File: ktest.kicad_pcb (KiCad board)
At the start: 4 copper layers, 23.9 x 21.1 mm, 7 parts, among them J1 Conn_01x03_Pin

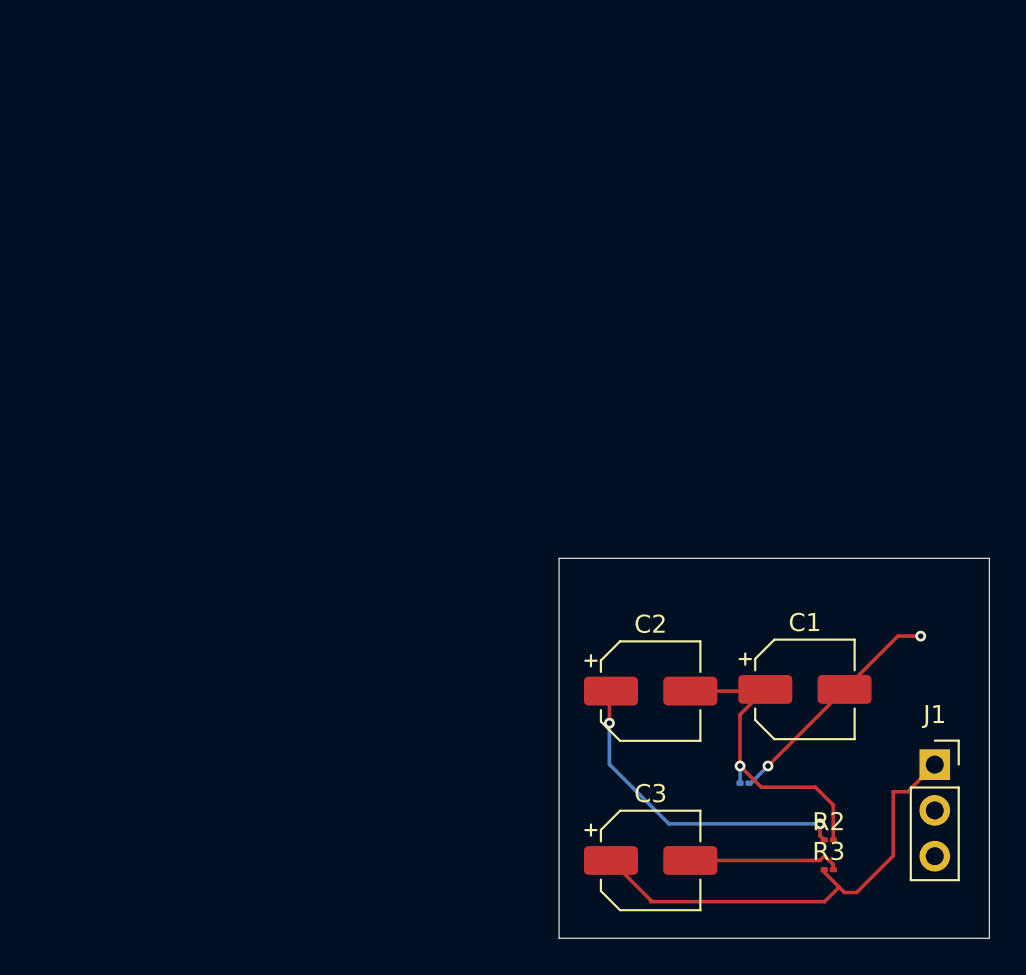
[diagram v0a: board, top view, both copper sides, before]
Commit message: Keep local changes
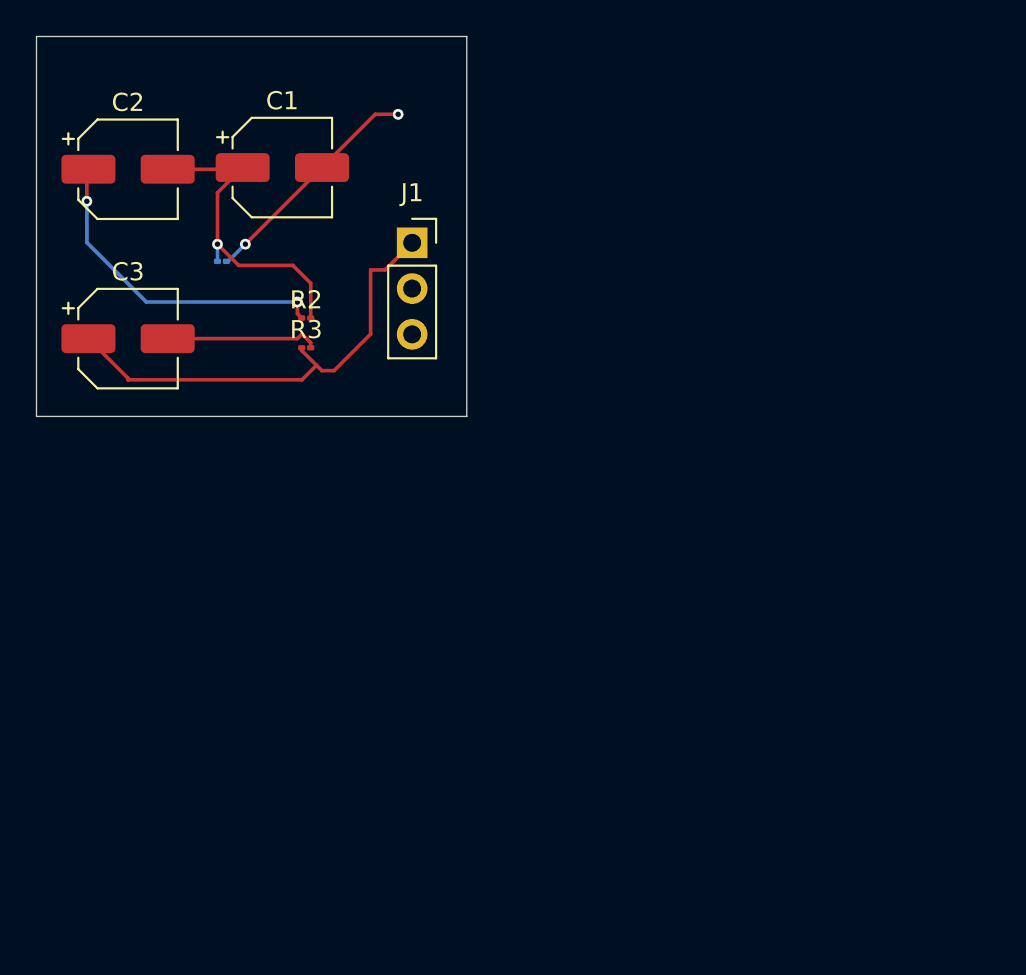
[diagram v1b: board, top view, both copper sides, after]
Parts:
- moved C2 41.0 mm to (97.5, 50.8)
- moved J1 41.0 mm to (113.3, 54.9)
- moved R1 41.0 mm to (102.7, 55.9)
- moved R2 41.0 mm to (107.4, 59.1)
- moved R3 41.0 mm to (107.4, 60.7)
- moved C3 41.0 mm to (97.5, 60.2)
- moved C1 41.0 mm to (106.1, 50.7)

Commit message: pdf assy image
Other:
- board text added: "angled bottom render"
- board text added: "angled top render"
- board text added: "bottom render"
- board text added: "top render"
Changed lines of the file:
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@@
 		(43 "User.3" user)
 		(45 "User.4" user)
+		(47 "User.5" user "AssemblyOverview")
+		(49 "User.6" user "AssemblyTop")
+		(51 "User.7" user "AssemblyBottom")
+		(53 "User.8" user)
 	)
 	(setup
@@
 		(capping no)
 		(filling no)
+		(zone_defaults)
 		(pcbplotparams
 			(layerselection 0x00000000_00000000_55555555_5755f5ff)
@@
 		(layer "Edge.Cuts")
 	)
+	(gr_rect
+		(start 40.132 39.624)
+		(end 77.724 75.946)
+		(stroke
+			(width 0.1)
+			(type default)
+		)
+		(fill no)
+		(layer "User.5")
+	)
+	(gr_rect
+		(start 126.746 40.005)
+		(end 164.338 76.327)
+		(stroke
+			(width 0.1)
+			(type default)
+		)
+		(fill no)
+		(layer "User.5")
+	)
+	(gr_rect
+		(start 139.954 51.054)
+		(end 174.752 85.598)
+		(stroke
+			(width 0.1)
+			(type default)
+		)
+		(fill no)
+		(layer "User.6")
+	)
+	(gr_rect
+		(start 133.096 36.322)
+		(end 161.29 68.072)
+		(stroke
+			(width 0.1)
+			(type default)
+		)
+		(fill no)
+		(layer "User.7")
+	)
+	(gr_text "angled top render"
+		(at 58.674 42.926 0)
+		(layer "User.5")
+		(effects
+			(font
+				(size 1 1)
+				(thickness 0.15)
+			)
+			(justify bottom)
+		)
+	)
+	(gr_text "angled bottom render"
+		(at 145.288 43.307 0)
+		(layer "User.5")
+		(effects
+			(font
+				(size 1 1)
+				(thickness 0.15)
+			)
+			(justify bottom)
+		)
+	)
+	(gr_text "top render"
+		(at 153.924 53.594 0)
+		(layer "User.6")
+		(effects
+			(font
+				(size 1 1)
+				(thickness 0.15)
+			)
+			(justify left bottom)
+		)
+	)
+	(gr_text "bottom render"
+		(at 141.986 38.862 0)
+		(layer "User.7")
+		(effects
+			(font
+				(size 1 1)
+				(thickness 0.15)
+			)
+			(justify left bottom)
+		)
+	)
 	(segment
 		(start 106.892 58.819)
@@
 		)
 	)
+	(group "kibot_image_blender_angled_bottom"
+		(members "47a33e86-0a7b-4fb2-9f1a-8c1f9bbd8aef" "e0f4d6b7-6642-4f52-86d4-2c7661283d27")
+	)
+	(group "kibot_image_blender_angled_top"
+		(members "aadaafd9-59d6-406c-9e50-c65a85ec2e7b" "d245d129-484e-4480-aa49-d9efff5859e8")
+	)
+	(group "kibot_image_blender_top"
+		(members "3748c16f-f86b-4ed3-95e1-1cd301faa602" "54584b5a-66d1-40a4-a952-5988b66ec816")
+	)
+	(group "kibot_image_blender_bottom"
+		(members "60365628-61de-4015-826d-ef046bea2621" "ef773150-5c25-4b16-be8e-16da88ff3160")
+	)
 	(embedded_fonts no)
